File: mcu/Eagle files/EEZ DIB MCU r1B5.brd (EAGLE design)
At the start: 139 x 70 mm, 197 parts, among them IC1 TPD4E001DRLR, IC10 TPS61169DCKR, IC11 TPD4E001DRLR, IC12 TPA6205A1DGN, IC13 TPD4E001DRLR, IC14 TSC2007IPW, IC15 TPD4E001DRLR, IC16 DP83848CVV/NOPB, IC2 SN74LVC2G34DBVR, IC3 BTS3408G, IC4 STM32F769IGT6, IC5 LD1117ADT33TR, IC6 TPD4E001DRLR, IC7 IS42S16400J, IC8 AT24C256C-SSHL-B, IC9 TPS2051BDBVR, J1 503398-1892, J2 67803-8020, Q1 MMBT5551, SW1 TL1100CF160Q, SW2 PEC16-2215F-S0024, X1 ZL263-40DG, X2 ZL231-16KG, X3 1844249, X4 22-23-2061, X5 LMJTAB881243M-L, Y1 25MHz, Y2 XTAL016178-85SMX

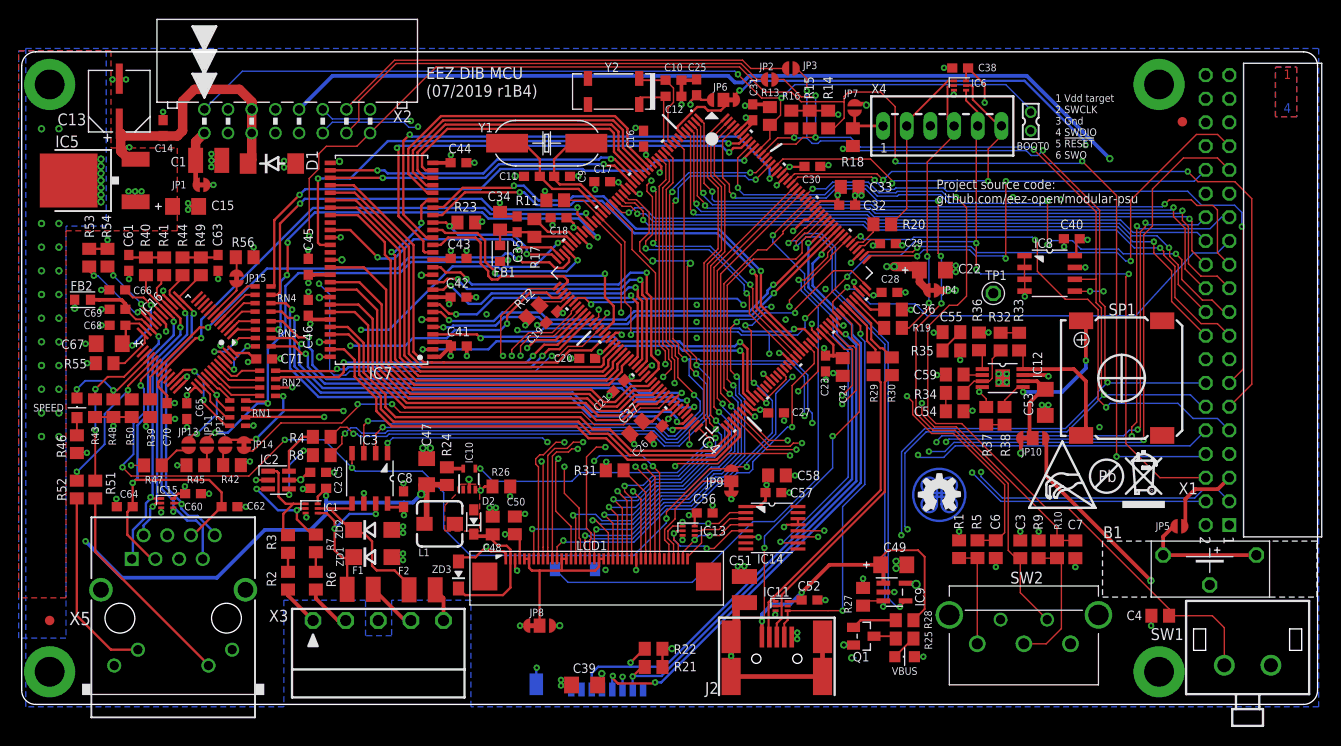
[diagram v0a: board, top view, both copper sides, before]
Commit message: #44, #45 Eagle files
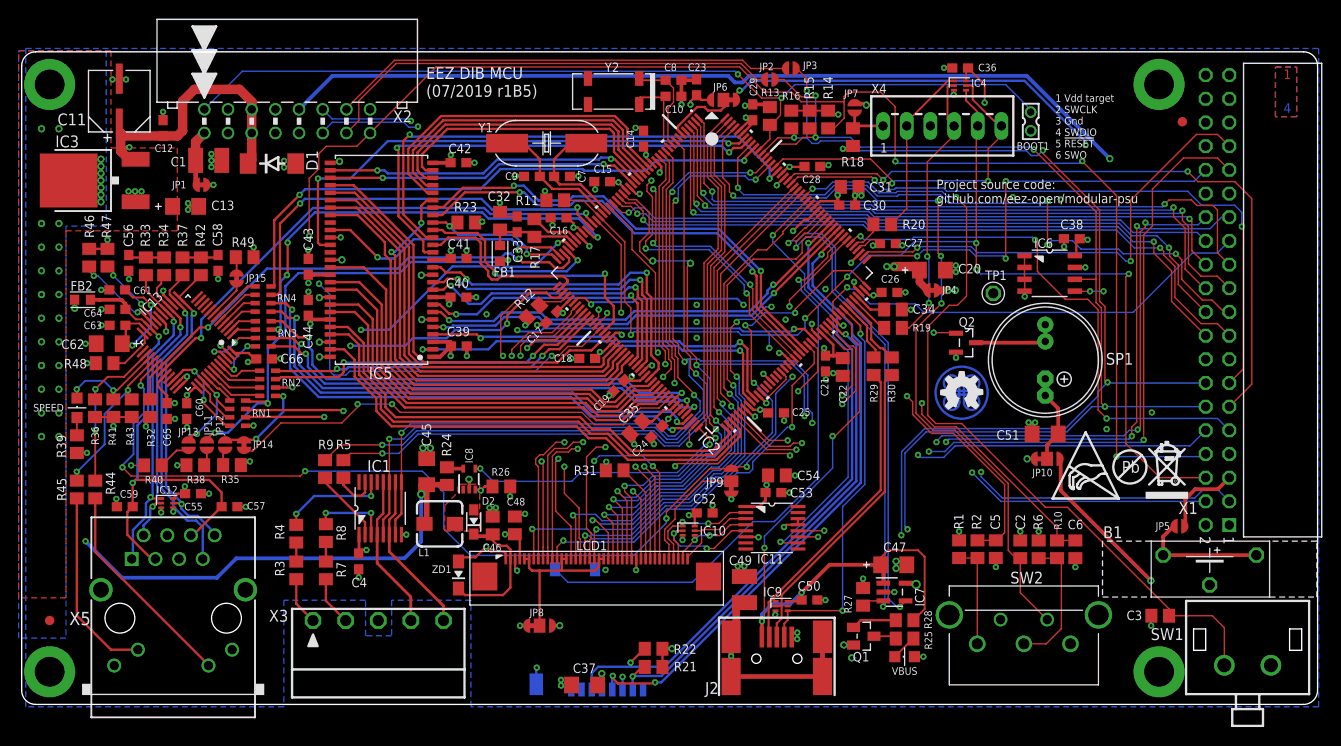
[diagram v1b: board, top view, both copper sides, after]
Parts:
- removed C67: 10u, EEZ_Lib1:EC1206
- removed C68, C69, C70, C71: 100n, rcl:C0603
- removed F1, F2: 50mA, EEZ_Lib1:F1210
- removed IC14: TSC2007IPW, EEZ_Lib1:PW(R-PDSO-G16)
- removed IC15: TPD4E001DRLR, EEZ_Lib1:DRL6
- removed IC16: DP83848CVV/NOPB, EEZ_Lib1:PT48
- removed R50, R53, R54, R56: 2K2, rcl:R0805
- removed R51, R52: 220R, rcl:R0805
- removed R55: 4K87, rcl:R0805
- removed ZD2: SMAJ18A, EEZ_Lib1:DO214AC
- removed ZD3: BZX384-B30.115, EEZ_Lib1:SOD323-W
- added Q2: 2N7002, EEZ_Lib1:SOT103P240X110-3N
- C11: value 18p -> EEEFK1V470P; device rcl:C0603 -> EEZ_Lib1:CAPAE660X610N
- C12: value 4p7 -> 100n
- C13: value EEEFK1V470P -> 4u7; device EEZ_Lib1:CAPAE660X610N -> EEZ_Lib1:EC1206
- C15: value 4u7 -> 100n; device EEZ_Lib1:EC1206 -> rcl:C0603
- C2, C5: value 100n -> 10n; device rcl:C0603 -> rcl:C0805
- C20: value 100n -> 4u7; device rcl:C0603 -> EEZ_Lib1:EC1206
- C22: value 4u7 -> 1u; device EEZ_Lib1:EC1206 -> rcl:C0805
- C23, C52: value 100n -> N.C.
- C24, C33, C58: value 1u -> 100n; device rcl:C0805 -> rcl:C0603
- C25: value N.C. -> 100n
- C31, C32, C46: value 100n -> 1u; device rcl:C0603 -> rcl:C0805
- C34, C48: value 1u -> 2u2
- C35: value 100n -> 2u2; device rcl:C0603 -> rcl:C0805
- C36: value 2u2 -> N.C.; device rcl:C0805 -> rcl:C0603
- C37: value 2u2 -> 4u7; device rcl:C0805 -> rcl:C1206
- C39, C53: value 4u7 -> 100n; device rcl:C1206 -> rcl:C0603
- C4: value 10n -> 100n; device rcl:C0805 -> rcl:C0603
- C45: value 100n -> 4u7; device rcl:C0603 -> rcl:C1206
- C47: device rcl:C1206 -> EEZ_Lib1:EC1206
- C49: value 4u7 -> N.C.; device EEZ_Lib1:EC1206 -> rcl:C1210
- C50: value 2u2 -> 100n; device rcl:C0805 -> rcl:C0603
- C51: value N.C. -> 4u7; device rcl:C1210 -> rcl:C1206
- C54: value 470n -> 1u
- C55: value 470n -> N.C.; device rcl:C0805 -> rcl:C0603
- C59: value N.C. -> 100n; device rcl:C0805 -> rcl:C0603
- C62: value 100n -> 10u; device rcl:C0603 -> EEZ_Lib1:EC1206
- C7: value 10n -> 18p; device rcl:C0805 -> rcl:C0603
- C8: value 100n -> 4p7
- IC1: value TPD4E001DRLR -> CD74HC4050PWR; device EEZ_Lib1:DRL6 -> EEZ_DIB:PW16
- IC10: value TPS61169DCKR -> TPD4E001DRLR; device EEZ_Lib1:DCK5 -> EEZ_Lib1:DRL6
- IC11: value TPD4E001DRLR -> TSC2007IPW; device EEZ_Lib1:DRL6 -> EEZ_Lib1:PW(R-PDSO-G16)
- IC12: value TPA6205A1DGN -> TPD4E001DRLR; device EEZ_Lib1:SOP65P490X110-9N -> EEZ_Lib1:DRL6
- IC13: value TPD4E001DRLR -> DP83848CVV/NOPB; device EEZ_Lib1:DRL6 -> EEZ_Lib1:PT48
- IC2: value SN74LVC2G34DBVR -> STM32F769IGT6; device EEZ_Lib1:DBV6 -> EEZ_DIB:LQFP-176_24X24MM
- IC3: value BTS3408G -> LD1117ADT33TR; device EEZ_Lib1:SOIC127P600X173-8N -> v-reg:DPACK
- IC4: value STM32F769IGT6 -> TPD4E001DRLR; device EEZ_DIB:LQFP-176_24X24MM -> EEZ_Lib1:DRL6
- IC5: value LD1117ADT33TR -> IS42S16400J; device v-reg:DPACK -> EEZ_Lib1:TSOPII-54
- IC6: value TPD4E001DRLR -> AT24C256C-SSHL-B; device EEZ_Lib1:DRL6 -> EEZ_Lib1:SOIC127P600X173-8N
- IC7: value IS42S16400J -> TPS2051BDBVR; device EEZ_Lib1:TSOPII-54 -> EEZ_Lib1:DBV5
- IC8: value AT24C256C-SSHL-B -> TPS61169DCKR; device EEZ_Lib1:SOIC127P600X173-8N -> EEZ_Lib1:DCK5
- IC9: value TPS2051BDBVR -> TPD4E001DRLR; device EEZ_Lib1:DBV5 -> EEZ_Lib1:DRL6
- Q1: value MMBT5551 -> N.C.
- R18: value 10K -> N.C.
- R19, R20: value 22R -> N.C.
- R2: value 4K7 -> 10K
- R25: value 330R -> N.C.
- R28: value 47K -> N.C.
- R32: value 10K -> 1K5
- R33, R34, R37: value 10K -> 49R9
- R35, R38: value 10K -> 2K2
- R36: value 47K -> 2K2
- R39: value 1K5 -> N.C.
- R4, R8: value 1K -> 4K7
- R40, R41, R49: value 49R9 -> 2K2
- R42: value 2K2 -> 49R9
- R44: value 49R9 -> 220R
- R45: value 2K2 -> 220R
- R46: value 220R -> 2K2
- R48: value 2K2 -> 4K87
- R5: value 10K -> 1K
- R9: value 4K7 -> 1K
- SP1: value LD-BZEL-M1313 -> AI-1223-TWT or LD-BZEN 0903; device EEZ_Lib1:LD-BZEL-M1313 -> EEZ_Lib1:AI-1223-TWT_COMBO
- SPEED: value LTST-C170YKT -> N.C.
- VBUS: value HSMG-C170 -> N.C.
- X4: value 22-23-2061 -> N.C.
- ZD1: value SMAJ18A -> BZX384-B30.115; device EEZ_Lib1:DO214AC -> EEZ_Lib1:SOD323-W
- moved R36 95.1 mm to (3.37, 31.8)
- moved R33 94.0 mm to (8.83, 47.0), turned to 270 degrees
- moved R32 91.5 mm to (9.27, 31.8)
- moved IC12 90.6 mm to (11.1, 21.6)
- moved C59 90.1 mm to (6.55, 21.2)
- moved R37 87.7 mm to (12.8, 47.0), turned to 270 degrees
- moved R38 87.0 mm to (14.1, 25.7), turned to 0 degrees
- moved C4 86.2 mm to (31.6, 15.3), turned to 270 degrees
- moved R34 85.9 mm to (10.8, 47.0), turned to 90 degrees
- moved C55 83.2 mm to (13.9, 22.6), turned to 0 degrees
- moved R35 78.1 mm to (18.1, 25.7)
- moved R6 77.6 mm to (104.6, 16.6), turned to 270 degrees
- moved R9 77.0 mm to (28.0, 25.2), turned to 90 degrees
- moved C2 75.6 mm to (102.6, 16.6), turned to 270 degrees
- moved R2 74.0 mm to (98.0, 16.6), turned to 270 degrees
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- renumbered BOOT0 to BOOT1
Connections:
- removed net !AUDIO_SHDN: IC12.1, R36.1
- removed net N$166: IC12.8, R33.1, SP1.-
- removed net N$171: IC12.4, R35.1, R37.2
- removed net N$181: IC12.3, R32.2, R34.1
- removed net N$193: C54.1, R34.2
- removed net N$194: C59.2, IC12.2
- removed net N$195: C55.1, R35.2
- removed net N$44: F1.1, X3.4
- removed net N$45: F2.1, X3.5
- removed net N$50: IC12.5, R38.1, SP1.+
- removed net N$6: R37.1, R38.2
- net !FAULT: now also IC2.58; no longer IC3.1, IC4.58
- net !RESET: now also IC13.29, IC2.31, IC4.4; no longer IC16.29, IC3.4, IC4.31, IC6.4
- net !USB_OTG_FS_OC: now also IC2.146, IC7.3; no longer IC4.146, IC9.3
- net +3V3: now also C13.+, C36.1, C37.1, C38.2, C4.1, C40.1, C48.1, C52.2, C53.2, C54.2, C55.1, C65.1, C66.1, IC1.1, IC10.6, IC11.1, IC12.6, IC13.32, IC13.48, IC3.4, IC4.6, IC5.1, IC5.14, IC5.27, IC5.3, IC5.43, IC5.49, IC5.9, IC6.8, R32.2, R36.1, R39.1, R40.1, R41.1, R49.1, R6.1; no longer C15.+, C38.1, C40.2, C45.1, C46.1, C5.1, C50.1, C56.2, C57.2, C58.2, C60.1, C70.1, C71.1, IC13.6, IC14.1, IC15.6, IC16.32, IC16.48, IC2.5, IC5.4, IC6.6, IC7.1, IC7.14, IC7.27, IC7.3, IC7.43, IC7.49, IC7.9, IC8.8, R36.2, R39.2, R48.1, R50.1, R53.1, R54.1, R56.1, R9.1
- net +3V3(A): now also C57.2, C59.2, C64.1, IC13.22; no longer C62.2, C64.2, C69.1, IC16.22
- net +5V: now also C11.1, C12.1, C45.1, IC3.3, IC7.5; no longer C13.1, C14.1, C2.1, C47.1, C8.2, IC1.6, IC3.8, IC5.3, IC9.5
- net BOOT0: now also IC2.166; no longer IC4.166
- net BYPASS_REG: now also IC2.48; no longer IC4.48
- net DAC_OUT1: now also IC2.50, Q2.1; no longer C55.2, IC4.50
- net DIN2: now also IC2.8, R9.2; no longer IC4.8, R8.2
- net DOUT2: now also IC1.7, IC1.9, IC2.163; no longer IC3.3, IC4.163
- net ENC_A: now also C5.2, IC2.119, R2.1; no longer C6.2, IC4.119, R5.1
- net ENC_B: now also C6.1, IC2.120; no longer C7.1, IC4.120
- net ENC_SW: now also C2.2, IC2.173; no longer C3.2, IC4.173
- net EOUT_A: now also R6.2; no longer R9.2
- net EOUT_B: now also R2.2; no longer R5.2
- net ETH_COL: now also IC2.47; no longer IC4.47
- net ETH_CRS: now also IC2.40; no longer IC4.40
- net ETH_MDC: now also IC13.31, IC2.33; no longer IC16.31, IC4.33
- net ETH_MDIO: now also IC13.30, IC2.42, R32.1; no longer IC16.30, IC4.42, R39.1
- net ETH_RXD0: now also IC2.54; no longer IC4.54
- net ETH_RXD1: now also IC2.55; no longer IC4.55
- net ETH_RXD2: now also IC2.83; no longer IC4.83
- net ETH_RXD3: now also IC2.84; no longer IC4.84
- net ETH_RX_CLK: now also IC2.41; no longer IC4.41
- net ETH_RX_DV: now also IC2.53; no longer IC4.53
- net ETH_RX_ERR: now also IC2.79; no longer IC4.79
- net ETH_TXD0: now also IC2.85; no longer IC4.85
- net ETH_TXD1: now also IC2.86; no longer IC4.86
- net ETH_TXD2: now also IC2.34; no longer IC4.34
- net ETH_TXD3: now also IC2.167; no longer IC4.167
- net ETH_TX_CLK: now also IC2.35; no longer IC4.35
- net ETH_TX_EN: now also IC2.80; no longer IC4.80
- net FMC_A0: now also IC2.16, IC5.23; no longer IC4.16, IC7.23
- net FMC_A1: now also IC2.17, IC5.24; no longer IC4.17, IC7.24
- net FMC_A10: now also IC2.66, IC5.22; no longer IC4.66, IC7.22
- net FMC_A11: now also IC2.67, IC5.35; no longer IC4.67, IC7.35
- net FMC_A2: now also IC2.18, IC5.25; no longer IC4.18, IC7.25
- net FMC_A3: now also IC2.19, IC5.26; no longer IC4.19, IC7.26
- net FMC_A4: now also IC2.20, IC5.29; no longer IC4.20, IC7.29
- net FMC_A5: now also IC2.21, IC5.30; no longer IC4.21, IC7.30
- net FMC_A6: now also IC2.60, IC5.31; no longer IC4.60, IC7.31
- net FMC_A7: now also IC2.63, IC5.32; no longer IC4.63, IC7.32
- net FMC_A8: now also IC2.64, IC5.33; no longer IC4.64, IC7.33
- net FMC_A9: now also IC2.65, IC5.34; no longer IC4.65, IC7.34
- net FMC_BA0: now also IC2.112, IC5.20; no longer IC4.112, IC7.20
- net FMC_BA1: now also IC2.113, IC5.21; no longer IC4.113, IC7.21
- net FMC_D0: now also IC2.97, IC5.2; no longer IC4.97, IC7.2
- net FMC_D1: now also IC2.98, IC5.4; no longer IC4.98, IC7.4
- net FMC_D10: now also IC2.76, IC5.45; no longer IC4.76, IC7.45
- net FMC_D11: now also IC2.77, IC5.47; no longer IC4.77, IC7.47
- net FMC_D12: now also IC2.78, IC5.48; no longer IC4.78, IC7.48
- net FMC_D13: now also IC2.89, IC5.50; no longer IC4.89, IC7.50
- net FMC_D14: now also IC2.90, IC5.51; no longer IC4.90, IC7.51
- net FMC_D15: now also IC2.91, IC5.53; no longer IC4.91, IC7.53
- net FMC_D2: now also IC2.142, IC5.5; no longer IC4.142, IC7.5
- net FMC_D3: now also IC2.143, IC5.7; no longer IC4.143, IC7.7
- net FMC_D4: now also IC2.68, IC5.8; no longer IC4.68, IC7.8
- net FMC_D5: now also IC2.69, IC5.10; no longer IC4.69, IC7.10
- net FMC_D6: now also IC2.70, IC5.11; no longer IC4.70, IC7.11
- net FMC_D7: now also IC2.73, IC5.13; no longer IC4.73, IC7.13
- net FMC_D8: now also IC2.74, IC5.42; no longer IC4.74, IC7.42
- net FMC_D9: now also IC2.75, IC5.44; no longer IC4.75, IC7.44
- net FMC_NBL0: now also IC2.169, IC5.15; no longer IC4.169, IC7.15
- net FMC_NBL1: now also IC2.170, IC5.39; no longer IC4.170, IC7.39
- net FMC_SDCKE0: now also IC2.43, IC5.37; no longer IC4.43, IC7.37
- net FMC_SDCLK: now also IC2.116, IC5.38; no longer IC4.116, IC7.38
- net FMC_SDNCAS: now also IC2.160, IC5.17; no longer IC4.160, IC7.17
- net FMC_SDNE0: now also IC2.44, IC5.19; no longer IC4.44, IC7.19
- net FMC_SDNRAS: now also IC2.59, IC5.18; no longer IC4.59, IC7.18
- net FMC_SDNWE: now also IC2.46, IC5.16; no longer IC4.46, IC7.16
- net GND: now also C11.2, C13.-, C15.2, C2.1, C20.-, C22.2, C38.1, C4.2, C40.2, C47.-, C49.2, C5.1, C50.1, C51.1, C54.1, C55.2, C56.2, C58.2, C6.2, C62.-, C64.2, C7.1, C8.2, IC1.8, IC10.3, IC11.13, IC11.14, IC11.6, IC12.3, IC13.15, IC13.19, IC13.35, IC13.36, IC13.47, IC2.103, IC2.109, IC2.117, IC2.130, IC2.135, IC2.14, IC2.148, IC2.158, IC2.22, IC2.37, IC2.61, IC2.71, IC2.95, IC3.1, IC4.3, IC5.12, IC5.28, IC5.41, IC5.46, IC5.52, IC5.54, IC5.6, IC6.1, IC6.2, IC6.4, IC6.7, IC7.2, IC9.3, Q2.2, R35.1, R38.1, R48.1; no longer C11.1, C13.2, C15.-, C2.2, C20.2, C22.-, C38.2, C4.1, C40.1, C47.2, C49.-, C5.2, C50.2, C51.2, C54.2, C56.1, C58.1, C6.1, C62.1, C64.1, C67.-, C68.2, C69.2, C7.2, C70.2, C71.2, C8.1, IC1.3, IC10.2, IC11.3, IC12.7, IC12.TP, IC13.3, IC14.13, IC14.14, IC14.6, IC15.3, IC16.15, IC16.19, IC16.35, IC16.36, IC16.47, IC2.2, IC3.6, IC4.103, IC4.109, IC4.117, IC4.130, IC4.135, IC4.14, IC4.148, IC4.158, IC4.22, IC4.37, IC4.61, IC4.71, IC4.95, IC5.1, IC7.12, IC7.28, IC7.41, IC7.46, IC7.52, IC7.54, IC7.6, IC8.1, IC8.3, IC8.4, IC8.7, IC9.2, R42.1, R45.1, R55.1, ZD1.A, ZD2.A
- net I2C1_SCL: now also IC11.12, IC2.164, IC6.6; no longer IC14.12, IC4.164, IC8.6
- net I2C1_SDA: now also IC11.11, IC2.165, IC6.5; no longer IC14.11, IC4.165, IC8.5
- net IRQ_TOUCH: now also IC11.10, IC2.151; no longer IC14.10, IC4.151
- net LED_ACT: now also IC13.26, R36.2, R44.2; no longer IC16.26, R43.2, R51.2
- net LED_LINK: now also IC13.28, R43.2, R45.2; no longer IC16.28, R50.2, R52.2
- net LED_SPEED: now also IC13.27, R41.2; no longer IC16.27, R48.2
- net LTDC_B2: now also IC2.150; no longer IC4.150
- net LTDC_B3: now also IC2.154; no longer IC4.154
- net LTDC_B4: now also IC2.155; no longer IC4.155
- net LTDC_B5: now also IC2.174; no longer IC4.174
- net LTDC_B6: now also IC2.175; no longer IC4.175
- net LTDC_B7: now also IC2.176; no longer IC4.176
- net LTDC_CLK: now also IC2.115; no longer IC4.115
- net LTDC_DE: now also IC2.28; no longer IC4.28
- net LTDC_G2: now also IC2.52; no longer IC4.52
- net LTDC_G3: now also IC2.153; no longer IC4.153
- net LTDC_G4: now also IC2.45; no longer IC4.45
- net LTDC_G5: now also IC2.132; no longer IC4.132
- net LTDC_G6: now also IC2.13; no longer IC4.13
- net LTDC_G7: now also IC2.145; no longer IC4.145
- net LTDC_HSYNC: now also IC2.12; no longer IC4.12
- net LTDC_R2: now also IC2.139; no longer IC4.139
- net LTDC_R3: now also IC2.56; no longer IC4.56
- net LTDC_R4: now also IC2.51; no longer IC4.51
- net LTDC_R5: now also IC2.32; no longer IC4.32
- net LTDC_R6: now also IC2.57; no longer IC4.57
- net LTDC_R7: now also IC2.114; no longer IC4.114
- net LTDC_VSYNC: now also IC2.11; no longer IC4.11
- net MCLK_25: now also IC2.122; no longer IC4.122
- net N$1: now also IC13.1; no longer IC16.1
- net N$10: now also IC13.2; no longer IC16.2
- net N$101: now also R39.2; no longer R46.2
- net N$102: now also C58.1, R37.1, R42.2; no longer C63.1, R44.1, R49.2
- net N$11: now also IC13.39; no longer IC16.39
- net N$12: now also IC13.38; no longer IC16.38
- net N$15: now also IC13.3; no longer IC16.3
- net N$17: now also IC13.4; no longer IC16.4
- net N$178: now also IC2.100, IC2.106; no longer IC4.100, IC4.106
- net N$21: now also IC13.5; no longer IC16.5
- net N$22: now also IC13.34; no longer IC16.34
- net N$23: now also R40.2; no longer R47.2
- net N$25: now also R38.2; no longer R45.2
- net N$26: now also R35.2; no longer R42.2
- net N$27: now also IC13.7; no longer IC16.7
- net N$28: now also R49.2; no longer R56.2
- net N$29: now also IC13.6; no longer IC16.6
- net N$3: now also C56.1, R33.1, R34.2; no longer C61.1, R40.1, R41.2
- net N$30: now also IC8.5; no longer IC10.5
- net N$31: now also IC13.46; no longer IC16.46
- net N$32: now also IC13.45; no longer IC16.45
- net N$33: now also IC13.42; no longer IC16.42
- net N$34: now also IC13.44; no longer IC16.44
- net N$35: now also IC13.43; no longer IC16.43
- net N$36: now also IC13.41; no longer IC16.41
- net N$37: now also IC13.40; no longer IC16.40
- net N$38: now also R3.2, R4.1; no longer R2.2, R3.1
- net N$39: now also R3.1; no longer R2.1
- net N$40: now also R7.1; no longer R6.1
- net N$41: now also R7.2, R8.1; no longer R6.2, R7.1
- net N$42: now also IC1.15, R5.1; no longer IC2.6, R4.1
- net N$43: now also IC1.2, R9.1; no longer IC2.4, R8.1
- net N$46: now also IC1.14, R4.2; no longer IC1.1, IC2.1, R3.2
- net N$47: now also IC1.3, R8.2; no longer IC1.2, IC2.3, R7.2
- net N$48: now also IC1.12, X3.4; no longer F1.2, IC3.7, ZD1.C
- net N$49: now also IC1.10, IC1.6, X3.5; no longer F2.2, IC1.5, IC3.5, ZD2.C
- net N$5: now also Q2.3, SP1.-B, SP1.-B.1; no longer R32.1, R33.2
- net N$52: now also C51.2, SP1.+B, SP1.+B.1; no longer C53.2, IC12.6
- net N$8: now also R44.1; no longer R51.1
- net N$9: now also R45.1; no longer R52.1
- net N$97: now also IC13.24, R48.2; no longer IC16.24, R55.2
- net N$98: now also IC13.21, R46.2; no longer IC16.21, R53.2
- net N$99: now also IC13.20, R47.2; no longer IC16.20, R54.2
- net OE_SYNC: now also IC2.94; no longer IC4.94
- net PE: now also C49.1; no longer C51.1
- net PFBOUT: now also C60.1, C61.1, C62.+, C63.1, IC13.18, IC13.23, IC13.37; no longer C65.1, C66.1, C67.+, C68.1, IC16.18, IC16.23, IC16.37
- net PWR_DIRECT: now also IC2.110; no longer IC4.110
- net PWR_SSTART: now also IC2.111; no longer IC4.111
- net RCC_OSC32_IN: now also C8.1, IC2.9; no longer C10.1, IC4.9
- net RCC_OSC32_OUT: now also C10.1, IC2.10; no longer C12.1, IC4.10
- net RCC_OSC_IN: now also C7.2, IC2.29; no longer C9.2, IC4.29
- net RCC_OSC_OUT: now also C9.2, IC2.30; no longer C11.2, IC4.30
- net RD+: now also IC12.4, IC13.14, R37.2; no longer IC15.4, IC16.14, R44.2
- net RD-: now also IC12.5, IC13.13, R42.1; no longer IC15.5, IC16.13, R49.1
- net SDMMC1_CK: now also IC2.141; no longer IC4.141
- net SDMMC1_CMD: now also IC2.144; no longer IC4.144
- net SDMMC1_D0: now also IC2.121; no longer IC4.121
- net SD_DETECT: now also IC2.140; no longer IC4.140
- net SPI2_CLK: now also IC2.133; no longer IC4.133
- net SPI2_CSA: now also IC2.93; no longer IC4.93
- net SPI2_CSB: now also IC2.92; no longer IC4.92
- net SPI2_IRQ: now also IC2.123; no longer IC4.123
- net SPI2_MISO: now also IC2.87; no longer IC4.87
- net SPI2_MOSI: now also IC2.134; no longer IC4.134
- net SPI4_CLK: now also IC2.1; no longer IC4.1
- net SPI4_CSA: now also IC2.2; no longer IC4.2
- net SPI4_CSB: now also IC2.3; no longer IC4.3
- net SPI4_IRQ: now also IC2.168; no longer IC4.168
- net SPI4_MISO: now also IC2.4; no longer IC4.4
- net SPI4_MOSI: now also IC2.5; no longer IC4.5
- net SPI5_CLK: now also IC2.25; no longer IC4.25
- net SPI5_CSA: now also IC2.157; no longer IC4.157
- net SPI5_CSB: now also IC2.156; no longer IC4.156
- net SPI5_IRQ: now also IC2.138; no longer IC4.138
- net SPI5_MISO: now also IC2.26; no longer IC4.26
- net SPI5_MOSI: now also IC2.27; no longer IC4.27
- net SW_WLED: now also IC8.1; no longer IC10.1
- net SYS_JTCK-SWCLK: now also IC2.137; no longer IC4.137
- net SYS_JTDO-SWO: now also IC2.161, IC4.5; no longer IC4.161, IC6.5
- net SYS_JTMS-SWDIO: now also IC2.128; no longer IC4.128
- net TCK: now also IC4.1; no longer IC6.1
- net TD+: now also IC12.1, IC13.17, R33.2; no longer IC15.1, IC16.17, R40.2
- net TD-: now also IC12.2, IC13.16, R34.1; no longer IC15.2, IC16.16, R41.1
- net TFT_BRIGHTNESS: now also IC2.88, IC8.4; no longer IC10.4, IC4.88
- net TMS: now also IC4.2; no longer IC6.2
- net UART_RX/DIN1: now also IC2.24, R5.2; no longer IC4.24, R4.2
- net UART_TX/DOUT1: now also IC1.11, IC1.5, IC2.162; no longer IC3.2, IC4.162
- net USB_D_N: now also IC9.1; no longer IC11.1
- net USB_D_P: now also IC9.2; no longer IC11.2
- net USB_OTG_FS_D_N: now also IC2.126; no longer IC4.126
- net USB_OTG_FS_D_P: now also IC2.127; no longer IC4.127
- net USB_OTG_FS_ID: now also IC2.125, IC9.4; no longer IC11.4, IC4.125
- net USB_OTG_FS_PSO: now also IC2.147, IC7.4; no longer IC4.147, IC9.4
- net USB_OTG_FS_VBUS: now also C47.+, C50.2, IC2.124, IC7.1, IC9.6; no longer C49.+, C52.2, IC11.6, IC4.124, IC9.1
- net USER_SW: now also C3.2, IC2.152; no longer C4.2, IC4.152
- net VBAT: now also IC2.6; no longer IC4.6
- net VCAP1: now also C35.1, IC2.81; no longer C37.1, IC4.81
- net VCAP2: now also C34.1, IC2.129; no longer C36.1, IC4.129
- net VDD: now also C14.1, C15.1, C20.+, C22.1, IC2.118, IC2.131, IC2.136, IC2.149, IC2.15, IC2.159, IC2.171, IC2.172, IC2.23, IC2.36, IC2.49, IC2.62, IC2.72, IC2.82, IC2.96, IC2.99; no longer C20.1, C22.+, C32.1, C33.1, IC4.118, IC4.131, IC4.136, IC4.149, IC4.15, IC4.159, IC4.171, IC4.172, IC4.23, IC4.36, IC4.49, IC4.62, IC4.72, IC4.82, IC4.96, IC4.99
- net VDDA: now also C32.1, C33.1, IC2.39; no longer C34.1, C35.1, IC4.39
- net VLED+: now also C46.1, ZD1.C; no longer C48.1, ZD3.C
- net VLED-: now also IC8.3, ZD1.A; no longer IC10.3, ZD3.A
- net VREF+: now also IC2.38; no longer IC4.38
- net XL: now also IC10.4, IC11.4; no longer IC13.4, IC14.4
- net XR: now also IC10.1, IC11.2; no longer IC13.1, IC14.2
- net YD: now also IC10.2, IC11.5; no longer IC13.2, IC14.5
- net YU: now also IC10.5, IC11.3; no longer IC13.5, IC14.3
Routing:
- net !FAULT: track 225.5 -> 197.4 mm, vias 8 -> 6
- net N$50: track 17.6 -> 0.00 mm, vias 2 -> 0
- net N$166: track 15.4 -> 0.00 mm
- net GND: track 151.2 -> 139.6 mm, vias 155 -> 142
- net +5V: track 247.8 -> 239.2 mm, vias 7 -> 5
- net N$171: track 8.43 -> 0.00 mm, vias 2 -> 0
- net UART_TX/DOUT1: track 142.2 -> 149.7 mm
- net N$5: track 1.98 -> 9.27 mm
- net N$181: track 7.16 -> 0.00 mm
- net N$44: track 5.42 -> 0.00 mm
- net !RESET: track 238.1 -> 233.7 mm, vias 14 -> 13
- net DOUT2: track 77.8 -> 82.1 mm
- net N$45: track 3.66 -> 0.00 mm
- net N$47: track 11.5 -> 8.40 mm
- net N$195: track 2.76 -> 0.00 mm
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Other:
- board text added: "EEZ DIB MCU (07/2019 r1B5)"
- board text removed: "EEZ DIB MCU (07/2019 r1B4)"
